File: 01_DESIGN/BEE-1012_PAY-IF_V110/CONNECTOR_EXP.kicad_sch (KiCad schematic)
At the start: 8 parts, among them J3 5040500991, J4 5040500891

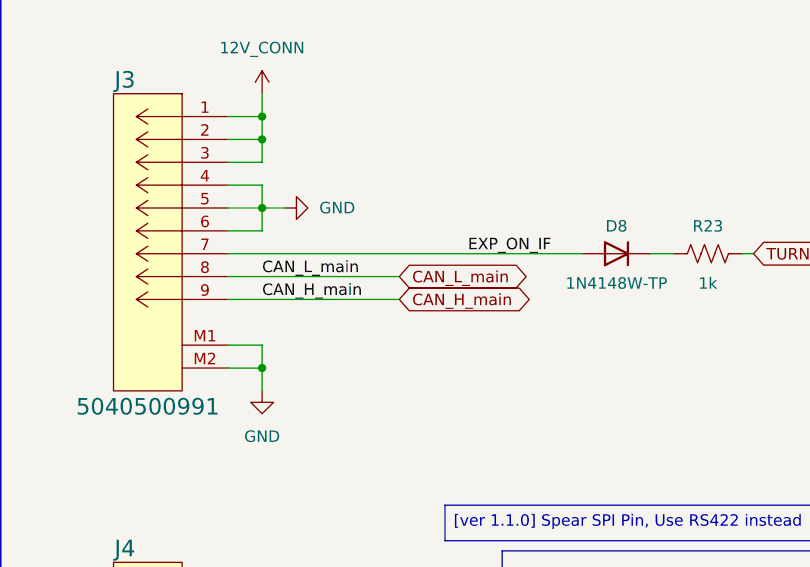
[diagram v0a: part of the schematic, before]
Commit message: Done Layout
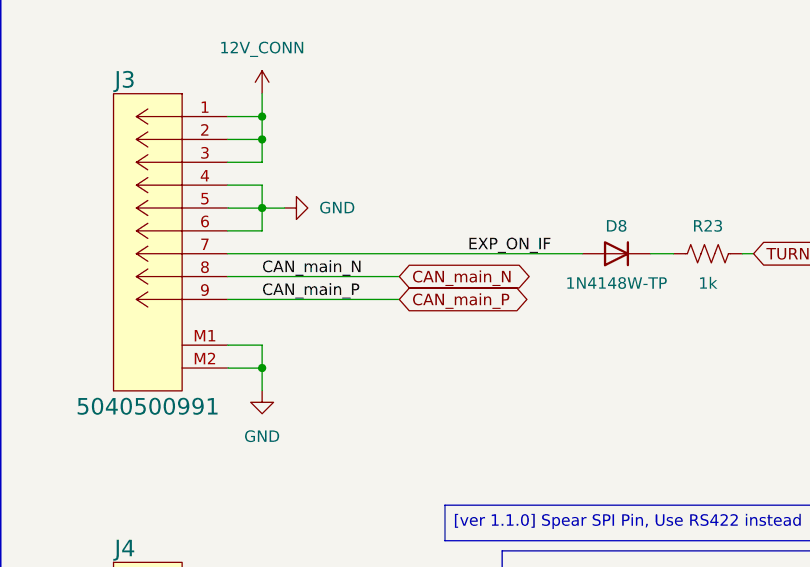
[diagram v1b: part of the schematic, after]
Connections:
- net CAN_H_main renamed CAN_main_P
- net CAN_L_main renamed CAN_main_N
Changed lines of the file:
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@@
 		)
 	)
-	(label "CAN_L_main"
+	(label "CAN_main_N"
 		(at 143.51 71.12 0)
 		(effects
@@
 		)
 	)
-	(label "CAN_H_main"
+	(label "CAN_main_P"
 		(at 143.51 73.66 0)
 		(effects
@@
 		)
 	)
-	(global_label "CAN_L_main"
+	(global_label "CAN_main_N"
 		(shape bidirectional)
 		(at 158.75 71.12 0)
@@
 		)
 		(property "Intersheetrefs" "${INTERSHEET_REFS}"
-			(at 174.095 71.12 0)
+			(at 174.3974 71.12 0)
 			(hide yes)
 			(show_name no)
@@
 		)
 	)
-	(global_label "CAN_H_main"
+	(global_label "CAN_main_P"
 		(shape bidirectional)
 		(at 158.75 73.66 0)
@@
 		)
 		(property "Intersheetrefs" "${INTERSHEET_REFS}"
-			(at 174.3974 73.66 0)
-			(hide yes)
-			(show_name no)
+			(at 174.3369 73.66 0)
+			(hide yes)
+			(show_name no)
